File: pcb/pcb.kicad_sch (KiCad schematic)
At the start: 2 parts

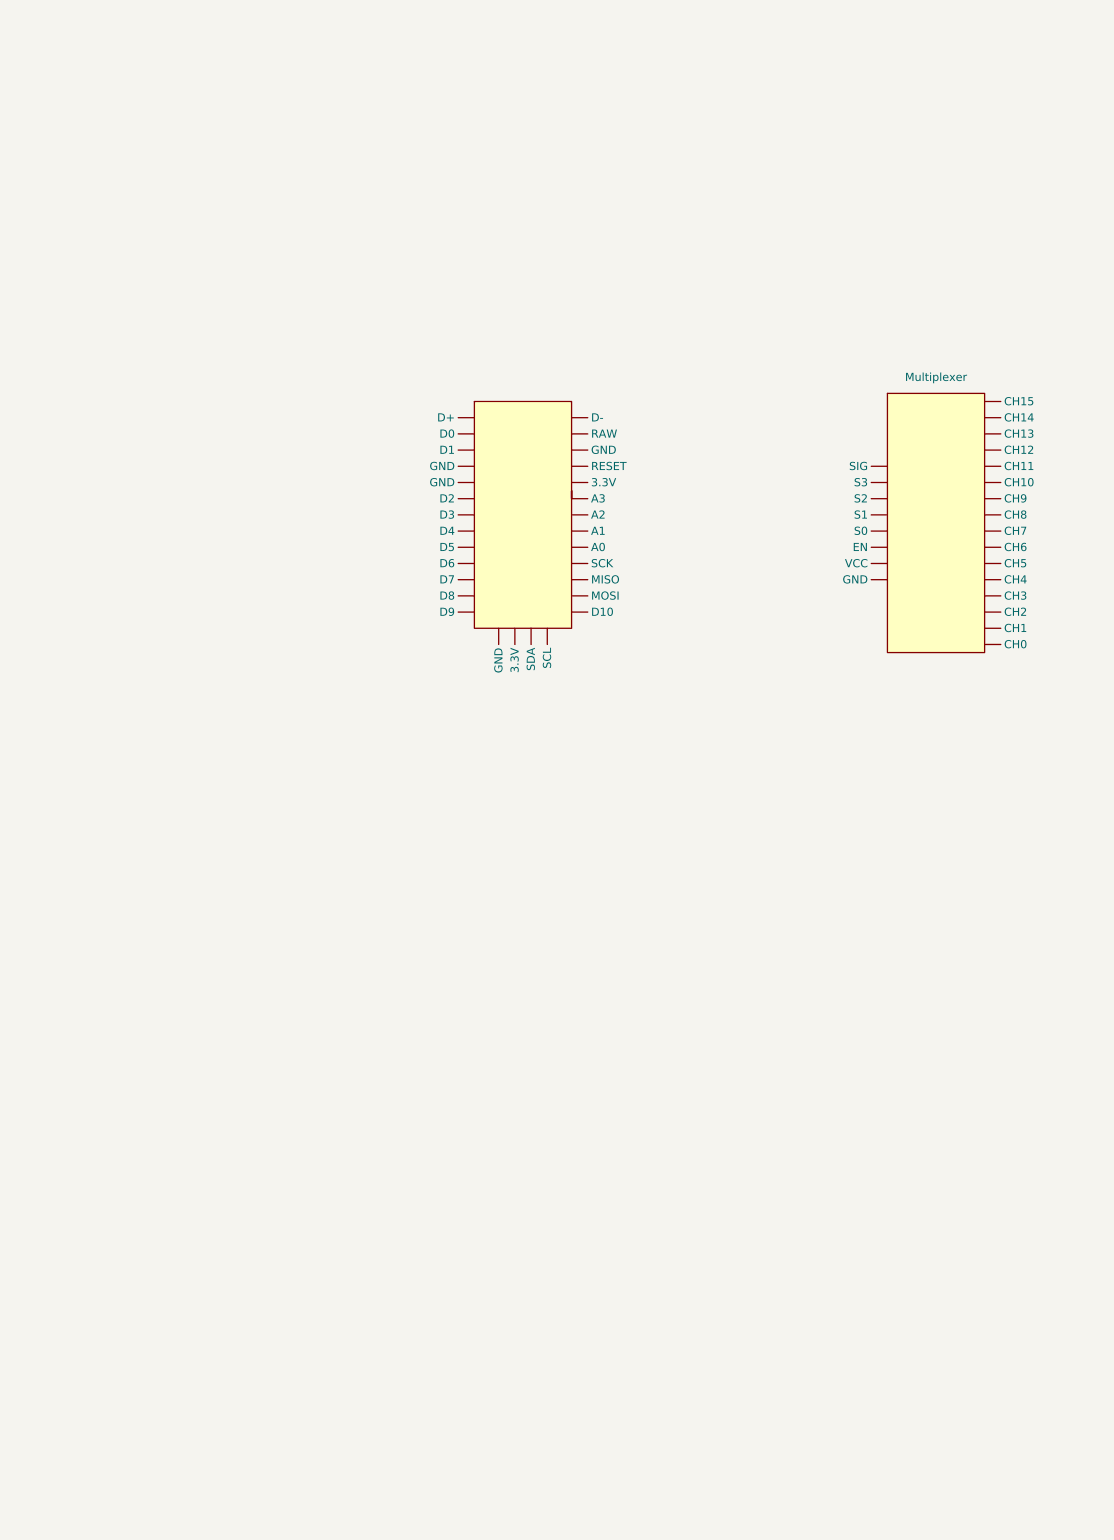
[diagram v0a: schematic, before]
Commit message: pcb schema
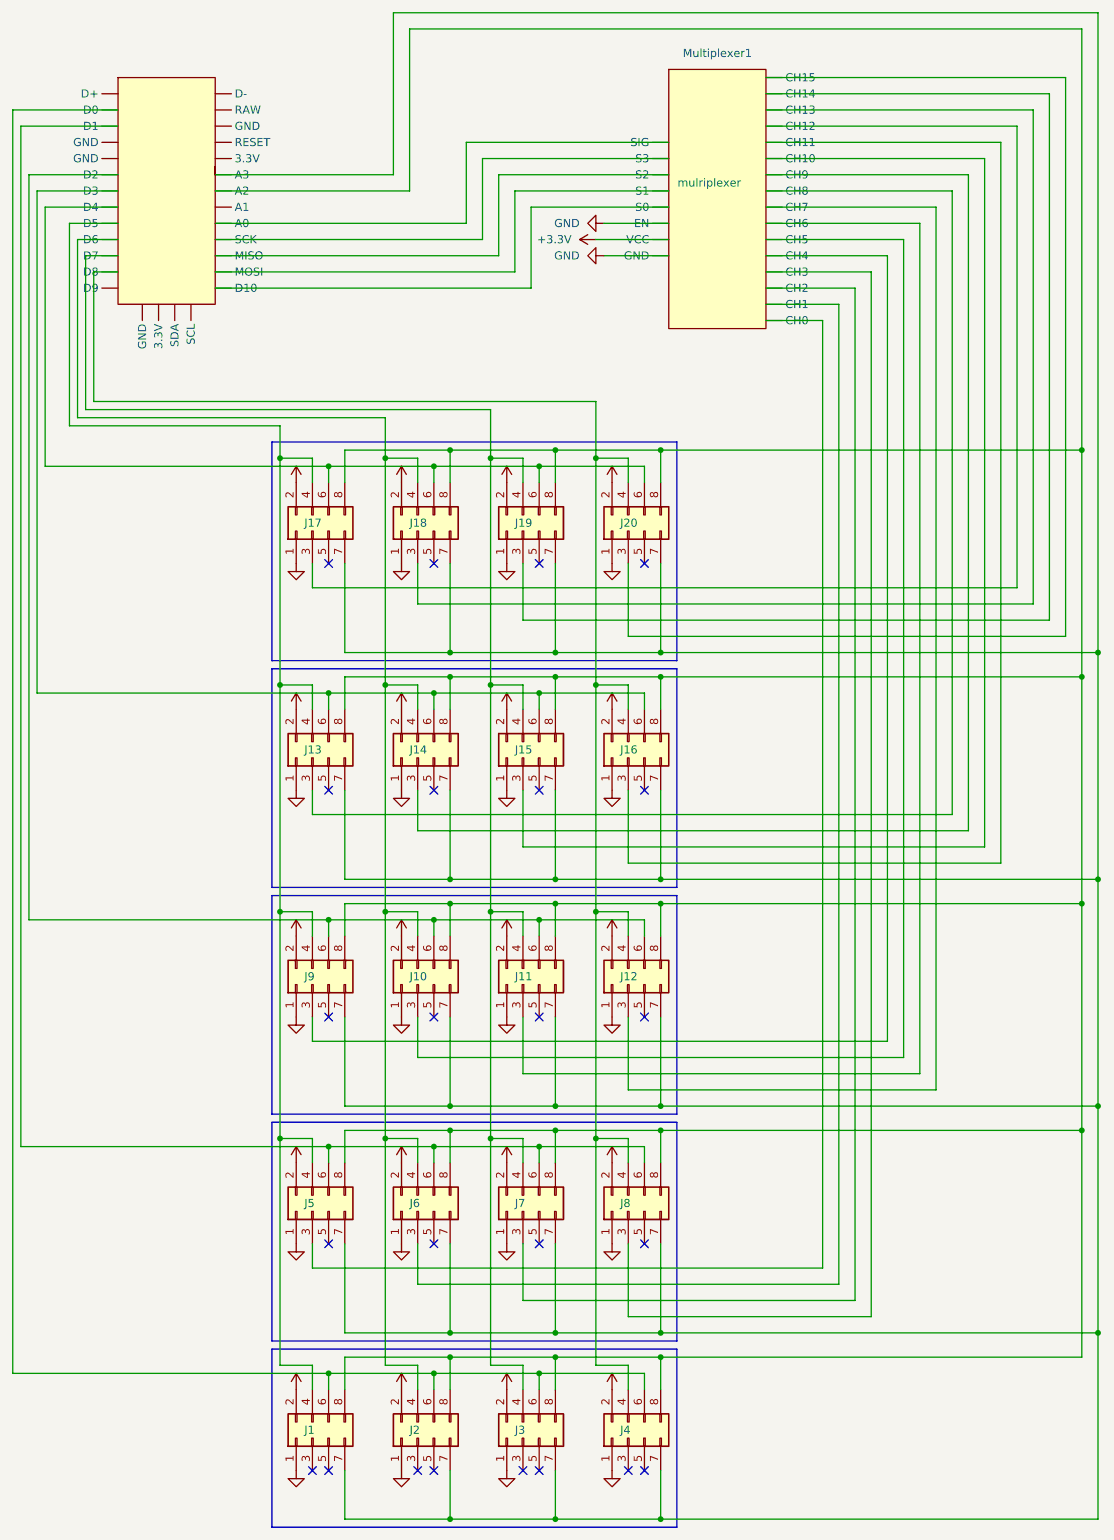
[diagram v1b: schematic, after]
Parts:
- added J1, J10, J11, J12, J13, J14, J15, J16, J17, J18, J19, J2, J20, J3, J4, J5, J6, J7, J8, J9: Conn_02x04_Odd_Even, symbol Connector_Generic:Conn_02x04_Odd_Even
- Multiplexer1: renamed from Multiplexer; value ~ -> mulriplexer
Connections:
- net at KB2040. (SDA): now also Multiplexer1. (VCC)
- net GND: now reaches Multiplexer1. (VCC)
- net GND: now also J1.1 (Pin_1), J10.1 (Pin_1), J11.1 (Pin_1), J12.1 (Pin_1), J13.1 (Pin_1), J14.1 (Pin_1), J15.1 (Pin_1), J16.1 (Pin_1), J17.1 (Pin_1), J18.1 (Pin_1), J19.1 (Pin_1), J2.1 (Pin_1), J20.1 (Pin_1), J3.1 (Pin_1), J4.1 (Pin_1), J5.1 (Pin_1), J6.1 (Pin_1), J7.1 (Pin_1), J8.1 (Pin_1), J9.1 (Pin_1)
- new net: J10.4 (Pin_4), J14.4 (Pin_4), J18.4 (Pin_4), J2.4 (Pin_4), J6.4 (Pin_4), KB2040. (SDA)
- new net: J13.6 (Pin_6), J14.6 (Pin_6), J15.6 (Pin_6), J16.6 (Pin_6), KB2040. (SDA)
- new net: J1.7 (Pin_7), J10.7 (Pin_7), J11.7 (Pin_7), J12.7 (Pin_7), J13.7 (Pin_7), J14.7 (Pin_7), J15.7 (Pin_7), J16.7 (Pin_7), J17.7 (Pin_7), J18.7 (Pin_7), J19.7 (Pin_7), J2.7 (Pin_7), J20.7 (Pin_7), J3.7 (Pin_7), J4.7 (Pin_7), J5.7 (Pin_7), J6.7 (Pin_7), J7.7 (Pin_7), J8.7 (Pin_7), J9.7 (Pin_7), KB2040. (SDA)
- new net: J1.8 (Pin_8), J10.8 (Pin_8), J11.8 (Pin_8), J12.8 (Pin_8), J13.8 (Pin_8), J14.8 (Pin_8), J15.8 (Pin_8), J16.8 (Pin_8), J17.8 (Pin_8), J18.8 (Pin_8), J19.8 (Pin_8), J2.8 (Pin_8), J20.8 (Pin_8), J3.8 (Pin_8), J4.8 (Pin_8), J5.8 (Pin_8), J6.8 (Pin_8), J7.8 (Pin_8), J8.8 (Pin_8), J9.8 (Pin_8), KB2040. (SDA)
- new net: J5.6 (Pin_6), J6.6 (Pin_6), J7.6 (Pin_6), J8.6 (Pin_6), KB2040. (SDA)
- new net: J10.6 (Pin_6), J11.6 (Pin_6), J12.6 (Pin_6), J9.6 (Pin_6), KB2040. (SDA)
- new net: J1.4 (Pin_4), J13.4 (Pin_4), J17.4 (Pin_4), J5.4 (Pin_4), J9.4 (Pin_4), KB2040. (SDA)
- new net: J12.4 (Pin_4), J16.4 (Pin_4), J20.4 (Pin_4), J4.4 (Pin_4), J8.4 (Pin_4), KB2040. (SDA)
- new net: J17.6 (Pin_6), J18.6 (Pin_6), J19.6 (Pin_6), J20.6 (Pin_6), KB2040. (SDA)
- new net: J1.6 (Pin_6), J2.6 (Pin_6), J3.6 (Pin_6), J4.6 (Pin_6), KB2040. (SDA)
- new net: J11.4 (Pin_4), J15.4 (Pin_4), J19.4 (Pin_4), J3.4 (Pin_4), J7.4 (Pin_4), KB2040. (SDA)
- new net: KB2040. (SDA), Multiplexer1. (VCC) (x4)
- new net: J14.3 (Pin_3), Multiplexer1. (VCC)
- new net: J6.3 (Pin_3), Multiplexer1. (VCC)
- new net: J10.3 (Pin_3), Multiplexer1. (VCC)
- new net: J5.3 (Pin_3), Multiplexer1. (VCC)
- new net: J12.3 (Pin_3), Multiplexer1. (VCC)
- new net: J20.3 (Pin_3), Multiplexer1. (VCC)
- new net: J13.3 (Pin_3), Multiplexer1. (VCC)
- new net: J18.3 (Pin_3), Multiplexer1. (VCC)
- new net: J7.3 (Pin_3), Multiplexer1. (VCC)
- new net: J11.3 (Pin_3), Multiplexer1. (VCC)
- new net: J17.3 (Pin_3), Multiplexer1. (VCC)
- new net: J16.3 (Pin_3), Multiplexer1. (VCC)
- new net: J15.3 (Pin_3), Multiplexer1. (VCC)
- new net: J9.3 (Pin_3), Multiplexer1. (VCC)
- new net: J8.3 (Pin_3), Multiplexer1. (VCC)
- new net: J19.3 (Pin_3), Multiplexer1. (VCC)
- new net +3.3V: J1.2 (Pin_2), J10.2 (Pin_2), J11.2 (Pin_2), J12.2 (Pin_2), J13.2 (Pin_2), J14.2 (Pin_2), J15.2 (Pin_2), J16.2 (Pin_2), J17.2 (Pin_2), J18.2 (Pin_2), J19.2 (Pin_2), J2.2 (Pin_2), J20.2 (Pin_2), J3.2 (Pin_2), J4.2 (Pin_2), J5.2 (Pin_2), J6.2 (Pin_2), J7.2 (Pin_2), J8.2 (Pin_2), J9.2 (Pin_2), Multiplexer1. (VCC)
- no-connect marks 0 -> 24
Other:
- moved on the sheet: Multiplexer1
